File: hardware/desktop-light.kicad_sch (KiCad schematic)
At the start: 82 parts, among them J1 Conn_01x06, J2 Conn_01x06, J3 USB_A, J4 Barrel_Jack, Q1 BSS138, Q2 BSS138, U1 ESP32-WROOM-32, U2 AMS1117-3.3, U3 CH340C

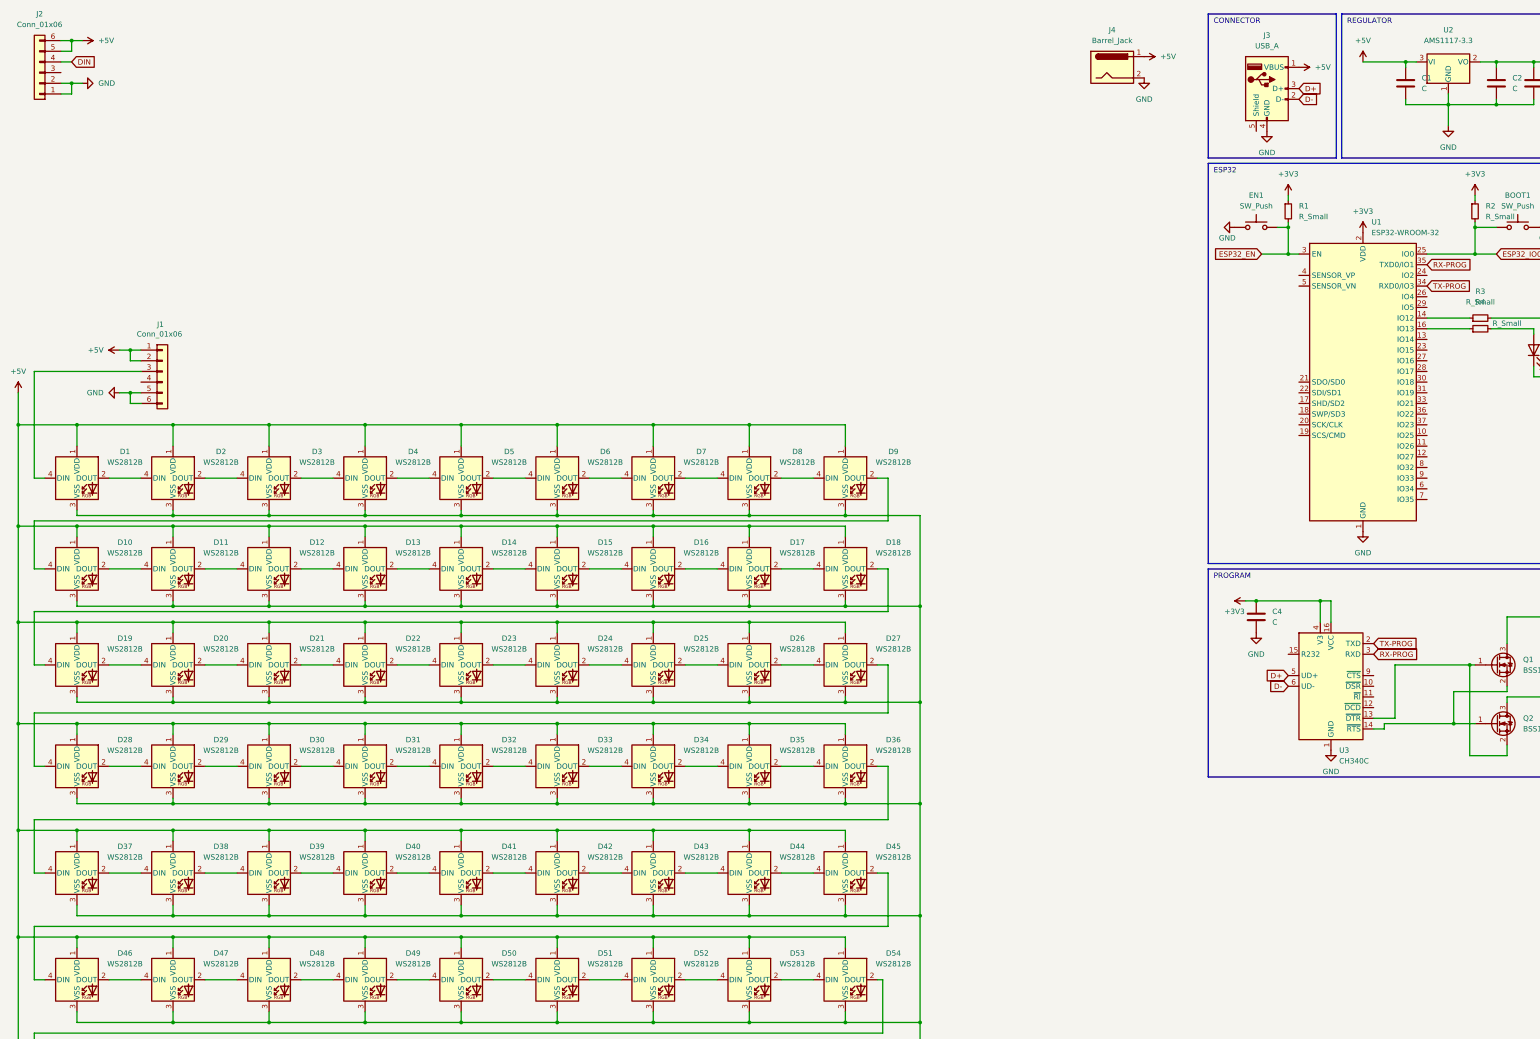
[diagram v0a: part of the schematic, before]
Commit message: add clock
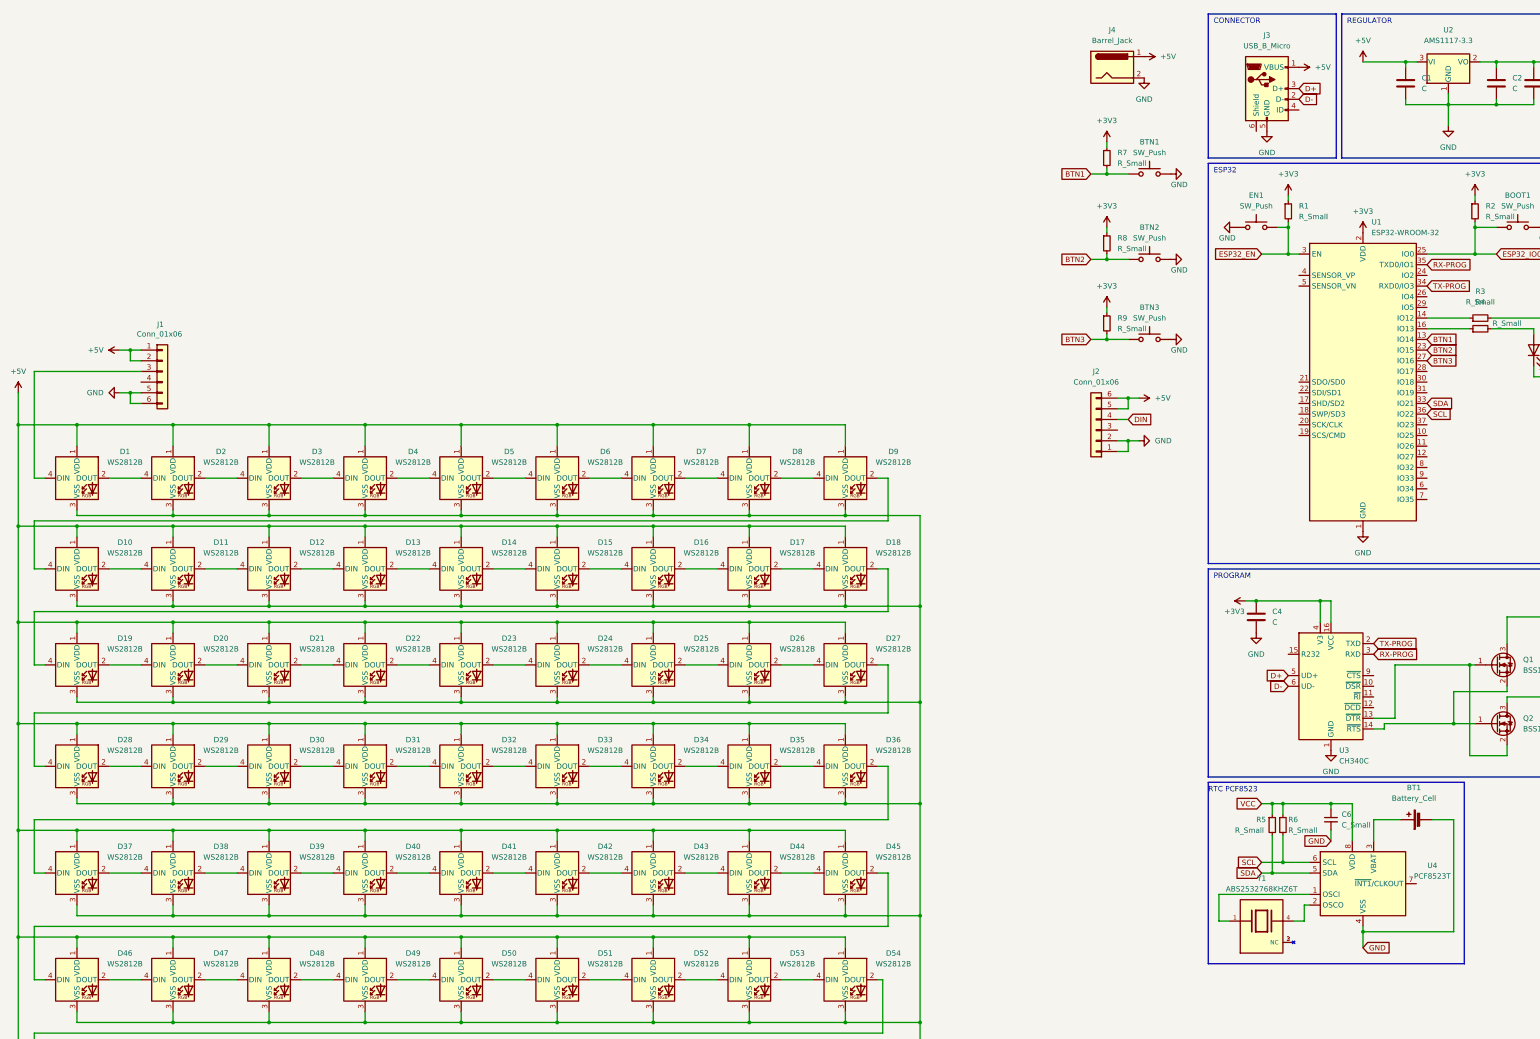
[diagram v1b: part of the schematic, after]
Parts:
- removed J3: USB_A, Connector_USB:USB_A_CNCTech_1001-011-01101_Horizontal, symbol Connector:USB_A
- added BT1: Battery_Cell, Battery:BatteryHolder_LINX_BAT-HLD-012-SMT, symbol Device:Battery_Cell
- added BTN1, BTN2, BTN3: SW_Push, Button_Switch_SMD:SW_SPST_FSMSM, symbol Switch:SW_Push
- added C6: C_Small, Capacitor_SMD:C_0603_1608Metric, symbol Device:C_Small
- added J3: USB_B_Micro, Connector_USB:USB_Micro-B_Molex-105017-0001, symbol Connector:USB_B_Micro
- added R5, R6, R7, R8, R9: R_Small, Resistor_SMD:R_0603_1608Metric, symbol Device:R_Small
- added U4: PCF8523T, Package_SO:SOIC-8_3.9x4.9mm_P1.27mm, symbol Timer_RTC:PCF8523T
- added Y1: ABS2532768KHZ6T, Crystal:Crystal_SMD_Abracon_ABS25-4Pin_8.0x3.8mm, symbol ABS2532768KHZ6T:ABS2532768KHZ6T
- J4: footprint (none) -> Connector_BarrelJack:BarrelJack_Wuerth_6941xx301002
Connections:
- net +3V3: now also R7.1, R8.1, R9.1
- net +5V: now also J3.1 (VBUS)
- net D+: now also J3.3 (D+)
- net D-: now also J3.2 (D-)
- net GND: now also BT1.2 (-), BTN1.2, BTN2.2, BTN3.2, C6.2, J3.5 (GND), U4.4 (VSS)
- net BTN1: now reaches U1.13 (IO14)
- net BTN1: now also BTN1.1, R7.2
- net BTN2: now reaches U1.23 (IO15)
- net BTN2: now also BTN2.1, R8.2
- net BTN3: now reaches U1.27 (IO16)
- net BTN3: now also BTN3.1, R9.2
- net SDA: now reaches U1.33 (IO21)
- net SDA: now also R5.2, U4.5 (SDA)
- net SCL: now reaches U1.36 (IO22)
- net SCL: now also R6.2, U4.6 (SCL)
- new net: U4.1 (OSCI), Y1.1
- new net: Y1.2 (NC), Y1.3 (NC)
- new net: U4.2 (OSCO), Y1.4
- new net: BT1.1 (+), U4.3 (VBAT)
- new net VCC: C6.1, R5.1, R6.1, U4.8 (VDD)
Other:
- note added: "RTC PCF8523"
- moved on the sheet: J2
